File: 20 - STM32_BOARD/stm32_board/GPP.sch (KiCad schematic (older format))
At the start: 2 parts, among them J1 Conn_01x04, J2 Conn_01x04

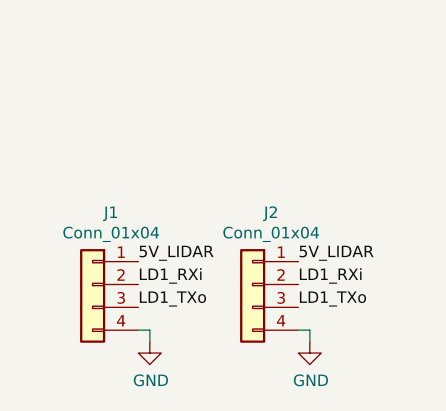
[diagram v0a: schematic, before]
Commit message: stm32
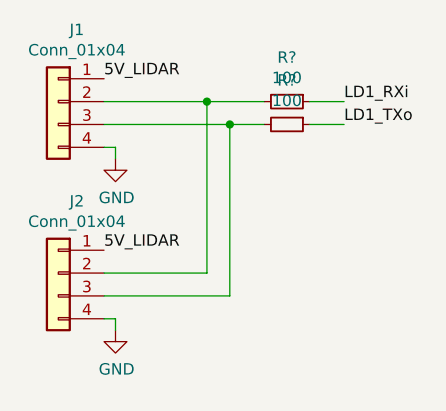
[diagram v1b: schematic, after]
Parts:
- added R? (x2): 100, symbol Device:R_Small
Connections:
- net LD1_RXi: now also R?.1; no longer J1.2 (Pin_2), J2.2 (Pin_2)
- net LD1_TXo: now also R?.1; no longer J1.3 (Pin_3), J2.3 (Pin_3)
- new net: J1.2 (Pin_2), J2.2 (Pin_2), R?.2
- new net: J1.3 (Pin_3), J2.3 (Pin_3), R?.2
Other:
- moved on the sheet: J1, J2
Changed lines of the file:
@@
 L Connector_Generic:Conn_01x04 J1
 U 1 1 5DA17A2F
-P 950 7200
-F 0 "J1" H 869 7514 50  0000 C CNN
-F 1 "Conn_01x04" H 869 7425 50  0000 C CNN
-F 2 "Connectors_JST:JST_SH_SM04B-SRSS-TB_04x1.00mm_Angled" H 950 7200 50  0001 C CNN
-F 3 "~" H 950 7200 50  0001 C CNN
-	1    950  7200
+P 800 6400
+F 0 "J1" H 719 6714 50  0000 C CNN
+F 1 "Conn_01x04" H 719 6625 50  0000 C CNN
+F 2 "Connectors_JST:JST_SH_SM04B-SRSS-TB_04x1.00mm_Angled" H 800 6400 50  0001 C CNN
+F 3 "~" H 800 6400 50  0001 C CNN
+	1    800  6400
 	-1   0    0    -1
 $EndComp
-Text Label 1150 7100 0    50   ~ 0
+Text Label 1000 6300 0    50   ~ 0
 5V_LIDAR
-Text Label 1150 7200 0    50   ~ 0
-LD1_RXi
-Text Label 1150 7300 0    50   ~ 0
-LD1_TXo
 $Comp
 L power:GND #PWR0101
 U 1 1 5DA196C0
-P 1200 7450
-F 0 "#PWR0101" H 1200 7200 50  0001 C CNN
-F 1 "GND" H 1205 7279 50  0000 C CNN
-F 2 "" H 1200 7450 50  0001 C CNN
-F 3 "" H 1200 7450 50  0001 C CNN
-	1    1200 7450
+P 1050 6650
+F 0 "#PWR0101" H 1050 6400 50  0001 C CNN
+F 1 "GND" H 1055 6479 50  0000 C CNN
+F 2 "" H 1050 6650 50  0001 C CNN
+F 3 "" H 1050 6650 50  0001 C CNN
+	1    1050 6650
 	1    0    0    -1
 $EndComp
 Wire Wire Line
-	1150 7400 1200 7400
+	1000 6600 1050 6600
 Wire Wire Line
-	1200 7400 1200 7450
+	1050 6600 1050 6650
 $Comp
 L Connector_Generic:Conn_01x04 J2
 U 1 1 5DA19F56
-P 1650 7200
-F 0 "J2" H 1569 7514 50  0000 C CNN
-F 1 "Conn_01x04" H 1569 7425 50  0000 C CNN
-F 2 "Pin_Headers:Pin_Header_Straight_1x04_Pitch2.54mm" H 1650 7200 50  0001 C CNN
-F 3 "~" H 1650 7200 50  0001 C CNN
-	1    1650 7200
+P 800 7150
+F 0 "J2" H 719 7464 50  0000 C CNN
+F 1 "Conn_01x04" H 719 7375 50  0000 C CNN
+F 2 "Pin_Headers:Pin_Header_Straight_1x04_Pitch2.54mm" H 800 7150 50  0001 C CNN
+F 3 "~" H 800 7150 50  0001 C CNN
+	1    800  7150
 	-1   0    0    -1
 $EndComp
-Text Label 1850 7100 0    50   ~ 0
+Text Label 1000 7050 0    50   ~ 0
 5V_LIDAR
-Text Label 1850 7200 0    50   ~ 0
+Text Label 2050 6400 0    50   ~ 0
 LD1_RXi
-Text Label 1850 7300 0    50   ~ 0
+Text Label 2050 6500 0    50   ~ 0
 LD1_TXo
 $Comp
 L power:GND #PWR0102
 U 1 1 5DA19F63
-P 1900 7450
-F 0 "#PWR0102" H 1900 7200 50  0001 C CNN
-F 1 "GND" H 1905 7279 50  0000 C CNN
-F 2 "" H 1900 7450 50  0001 C CNN
-F 3 "" H 1900 7450 50  0001 C CNN
-	1    1900 7450
+P 1050 7400
+F 0 "#PWR0102" H 1050 7150 50  0001 C CNN
+F 1 "GND" H 1055 7229 50  0000 C CNN
+F 2 "" H 1050 7400 50  0001 C CNN
+F 3 "" H 1050 7400 50  0001 C CNN
+	1    1050 7400
 	1    0    0    -1
 $EndComp
 Wire Wire Line
-	1850 7400 1900 7400
+	1000 7350 1050 7350
 Wire Wire Line
-	1900 7400 1900 7450
+	1050 7350 1050 7400
+$Comp
+L Device:R_Small R?
+U 1 1 5DA18202
+P 1800 6400
+F 0 "R?" V 1607 6400 50  0000 C CNN
+F 1 "100" V 1696 6400 50  0000 C CNN
+F 2 "" H 1800 6400 50  0001 C CNN
+F 3 "~" H 1800 6400 50  0001 C CNN
+	1    1800 6400
+	0    1    1    0
+$EndComp
+$Comp
+L Device:R_Small R?
+U 1 1 5DA19838
+P 1800 6500
+F 0 "R?" V 1607 6500 50  0000 C CNN
+F 1 "100" V 1696 6500 50  0000 C CNN
+F 2 "" H 1800 6500 50  0001 C CNN
+F 3 "~" H 1800 6500 50  0001 C CNN
+	1    1800 6500
+	0    1    1    0
+$EndComp
+Wire Wire Line
+	1000 6400 1450 6400
+Wire Wire Line
+	1000 6500 1550 6500
+Wire Wire Line
+	1450 7150 1450 6400
+Wire Wire Line
+	1000 7150 1450 7150
+Connection ~ 1450 6400
+Wire Wire Line
+	1450 6400 1700 6400
+Wire Wire Line
+	1550 7250 1550 6500
+Wire Wire Line
+	1000 7250 1550 7250
+Connection ~ 1550 6500
+Wire Wire Line
+	1550 6500 1700 6500
+Wire Wire Line
+	1900 6400 2050 6400
+Wire Wire Line
+	1900 6500 2050 6500
 $EndSCHEMATC

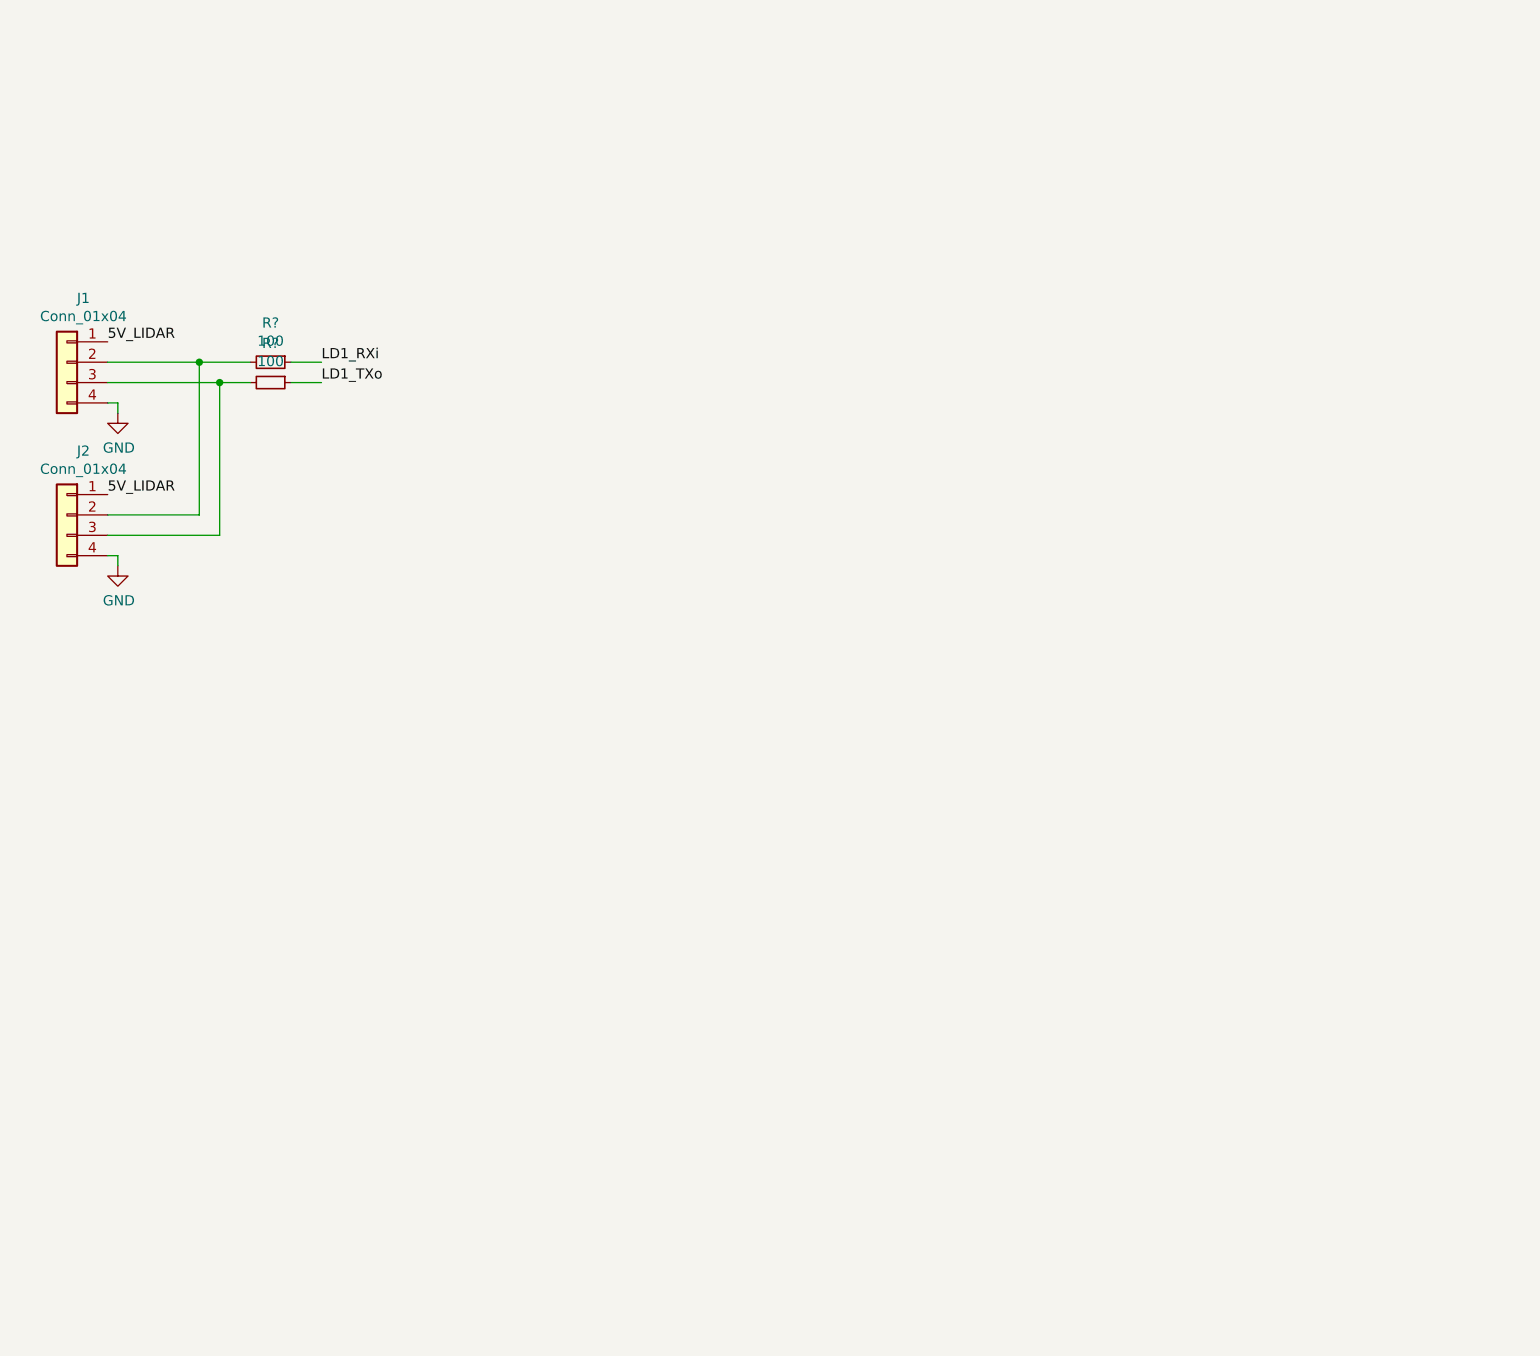
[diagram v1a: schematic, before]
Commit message: stm32
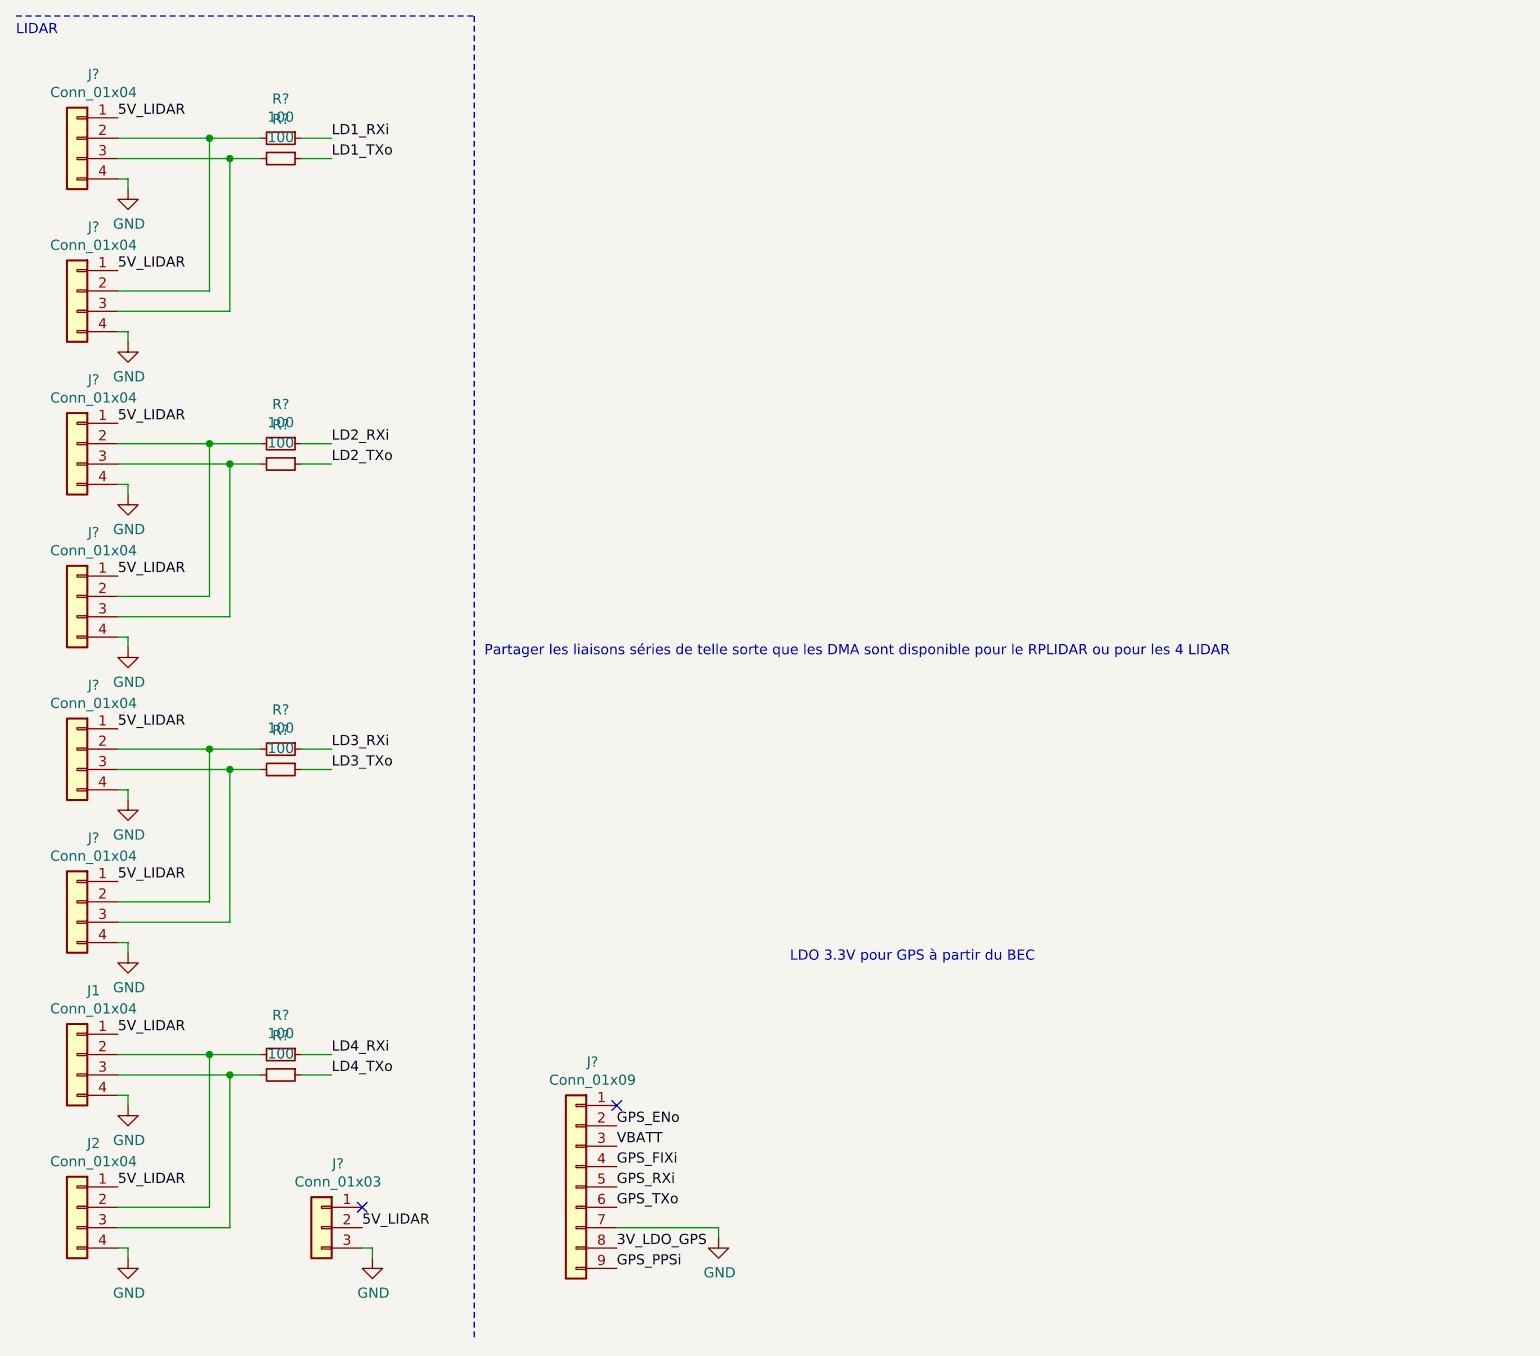
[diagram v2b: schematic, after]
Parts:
- added J? (x3): Conn_01x04, Connectors_JST:JST_SH_SM04B-SRSS-TB_04x1.00mm_Angled, symbol Connector_Generic:Conn_01x04
- added J? (x3): Conn_01x04, Pin_Headers:Pin_Header_Straight_1x04_Pitch2.54mm, symbol Connector_Generic:Conn_01x04
- added J?: Conn_01x03, symbol Connector_Generic:Conn_01x03
- added J?: Conn_01x09, symbol Connector_Generic:Conn_01x09
- added R? (x6): 100, symbol Device:R_Small
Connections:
- net 5V_LIDAR: now also J?.1 (Pin_1), J?.1 (Pin_1), J?.1 (Pin_1), J?.1 (Pin_1), J?.1 (Pin_1), J?.1 (Pin_1), J?.2 (Pin_2)
- net GND: now also J?.3 (Pin_3), J?.4 (Pin_4), J?.4 (Pin_4), J?.4 (Pin_4), J?.4 (Pin_4), J?.4 (Pin_4), J?.4 (Pin_4), J?.7 (Pin_7)
- net LD1_RXi: now also R?.1; no longer R?.1
- net LD1_TXo: now also R?.1; no longer R?.1
- new net: J?.2 (Pin_2), J?.2 (Pin_2), R?.2 (x3)
- new net: J?.3 (Pin_3), J?.3 (Pin_3), R?.2 (x3)
- new net 3V_LDO_GPS: J?.8 (Pin_8)
- new net GPS_ENo: J?.2 (Pin_2)
- new net GPS_FIXi: J?.4 (Pin_4)
- new net GPS_PPSi: J?.9 (Pin_9)
- new net GPS_RXi: J?.5 (Pin_5)
- new net GPS_TXo: J?.6 (Pin_6)
- new net LD2_RXi: R?.1
- new net LD2_TXo: R?.1
- new net LD3_RXi: R?.1
- new net LD3_TXo: R?.1
- new net LD4_RXi: R?.1
- new net LD4_TXo: R?.1
- new net VBATT: J?.3 (Pin_3)
- no-connect marks 0 -> 2
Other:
- note added: "LDO 3.3V pour GPS à partir du BEC"
- note added: "LIDAR"
- note added: "Partager les liaisons séries de telle sorte que les DMA sont disponible pour le RPLIDAR ou pour les 4 LIDAR"
- moved on the sheet: J1, J2, R?
